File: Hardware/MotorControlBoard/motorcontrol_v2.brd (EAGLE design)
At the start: 52.5 x 39 mm, 26 parts, among them U1 ATMEGA328P-AU

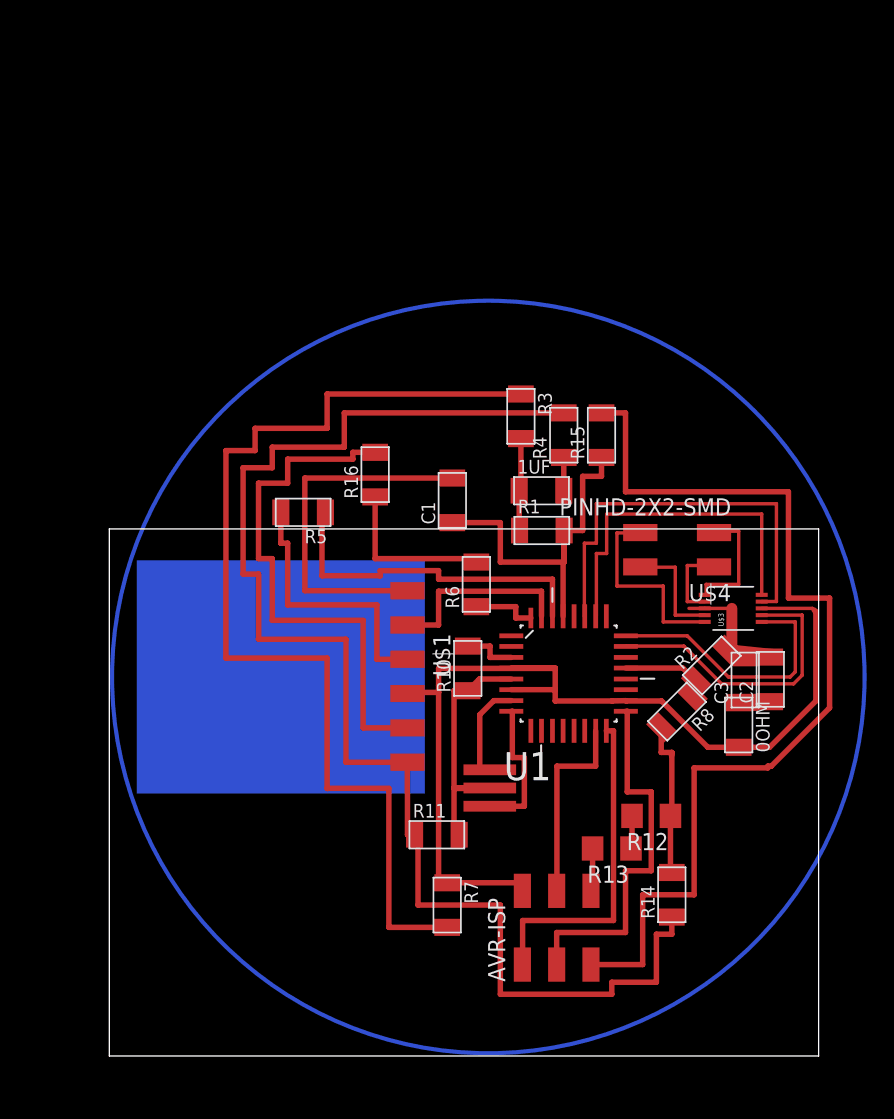
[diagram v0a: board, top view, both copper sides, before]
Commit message: new board stuff
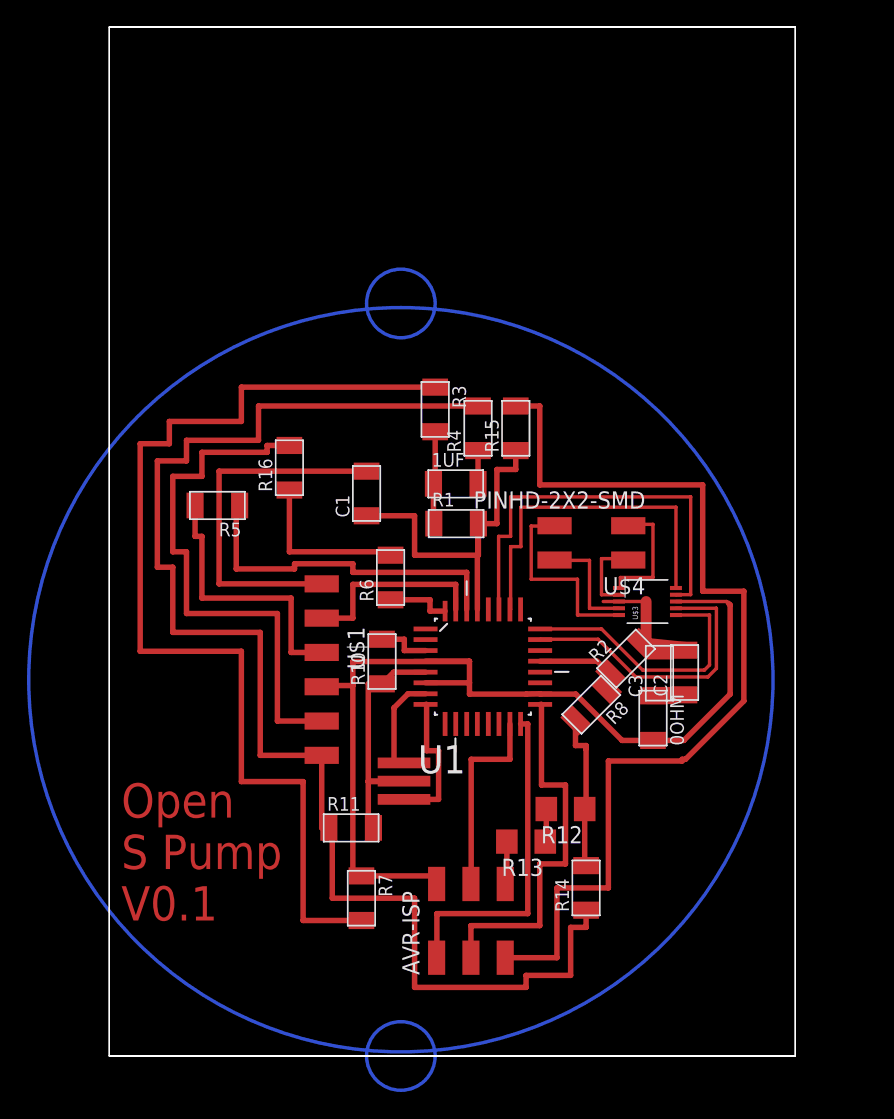
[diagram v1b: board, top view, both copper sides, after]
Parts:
- removed U$2: RESONATOR, fab:EFOBM
- added 20MHZ: 20MHZ, fab:EFOBM
- 0OHM, R5, R6: value (none) -> 0
- moved 0OHM 6.37 mm to (40.3, 25.0)
- moved C2 6.37 mm to (42.6, 28.4)
- moved C3 6.37 mm to (40.7, 28.3)
- moved R1 6.37 mm to (25.7, 39.4)
- moved R11 6.37 mm to (17.9, 16.9)
- moved R12 6.37 mm to (33.8, 18.3)
- moved R14 6.37 mm to (35.3, 12.4)
- moved R3 6.37 mm to (24.1, 47.9)
- moved R4 6.37 mm to (27.3, 46.5)
- moved R5 6.37 mm to (8.00, 40.8)
- moved R6 6.37 mm to (20.8, 35.4)
- moved R8 6.37 mm to (35.7, 26.0)
- moved U$4 6.37 mm to (35.9, 38.0)
- moved U$1 6.37 mm to (15.7, 28.6)
- moved 1UF 6.37 mm to (25.7, 42.4)
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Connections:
- net GNA: now also 20MHZ.2; no longer U$2.2
- net R1: now also 20MHZ.1; no longer U$2.1
- net R2: now also 20MHZ.3; no longer U$2.3
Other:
- board size 52.5 x 39 mm -> 50.8 x 76.2 mm
- board text added: "Open S Pump V0.1"

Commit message: lots of changes
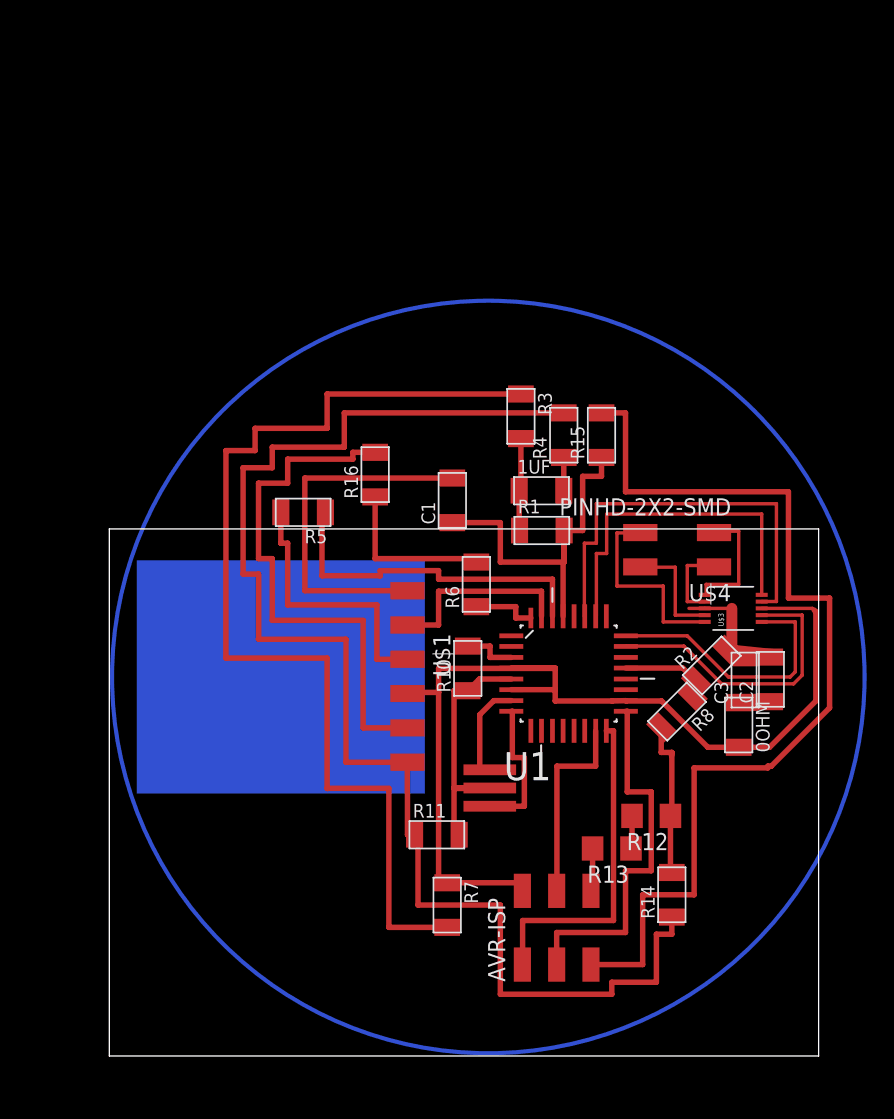
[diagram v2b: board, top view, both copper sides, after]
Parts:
- removed 20MHZ: 20MHZ, fab:EFOBM
- added U$2: RESONATOR, fab:EFOBM
- 0OHM, R5, R6: value 0 -> (none)
- moved 0OHM 6.37 mm to (46.6, 24.5)
- moved C2 6.37 mm to (48.9, 27.9)
- moved C3 6.37 mm to (47.1, 27.8)
- moved R1 6.37 mm to (32.0, 38.9)
- moved R11 6.37 mm to (24.3, 16.4)
- moved R12 6.37 mm to (40.1, 17.8)
- moved R14 6.37 mm to (41.7, 11.9)
- moved R3 6.37 mm to (30.5, 47.4)
- moved R4 6.37 mm to (33.7, 46.0)
- moved R5 6.37 mm to (14.4, 40.3)
- moved R6 6.37 mm to (27.2, 34.9)
- moved R8 6.37 mm to (42.0, 25.5)
- moved U$4 6.37 mm to (42.2, 37.5)
- moved U$1 6.37 mm to (22.1, 28.1)
- moved 1UF 6.37 mm to (32.0, 41.9)
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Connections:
- net GNA: now also U$2.2; no longer 20MHZ.2
- net R1: now also U$2.1; no longer 20MHZ.1
- net R2: now also U$2.3; no longer 20MHZ.3
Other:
- board size 50.8 x 76.2 mm -> 52.5 x 39 mm
- board text removed: "Open S Pump V0.1"
